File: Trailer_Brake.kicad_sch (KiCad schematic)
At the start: 11 parts, among them Q52 IRLZ44N, SW8 SW_SPST, U14 LM339

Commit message: Add files via upload
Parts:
- R201: footprint PCM_SL_Devices:Resistor_5W -> Resistor_THT:R_Axial_Power_L25.0mm_W9.0mm_P27.94mm
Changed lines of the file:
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@@
 			)
 		)
-		(property "Footprint" "PCM_SL_Devices:Resistor_5W"
+		(property "Footprint" "Resistor_THT:R_Axial_Power_L25.0mm_W9.0mm_P27.94mm"
 			(at 106.299 66.548 0)
 			(hide yes)

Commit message: Add files via upload
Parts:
- R202, R203: footprint (none) -> TRIM_3296W1103LF:TRIM_3296W1103LF
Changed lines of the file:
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@@
 			)
 		)
-		(property "Footprint" ""
+		(property "Footprint" "TRIM_3296W1103LF:TRIM_3296W1103LF"
 			(at 111.76 52.07 0)
 			(hide yes)
@@
 			)
 		)
-		(property "Footprint" ""
+		(property "Footprint" "TRIM_3296W1103LF:TRIM_3296W1103LF"
 			(at 123.19 73.66 0)
 			(hide yes)

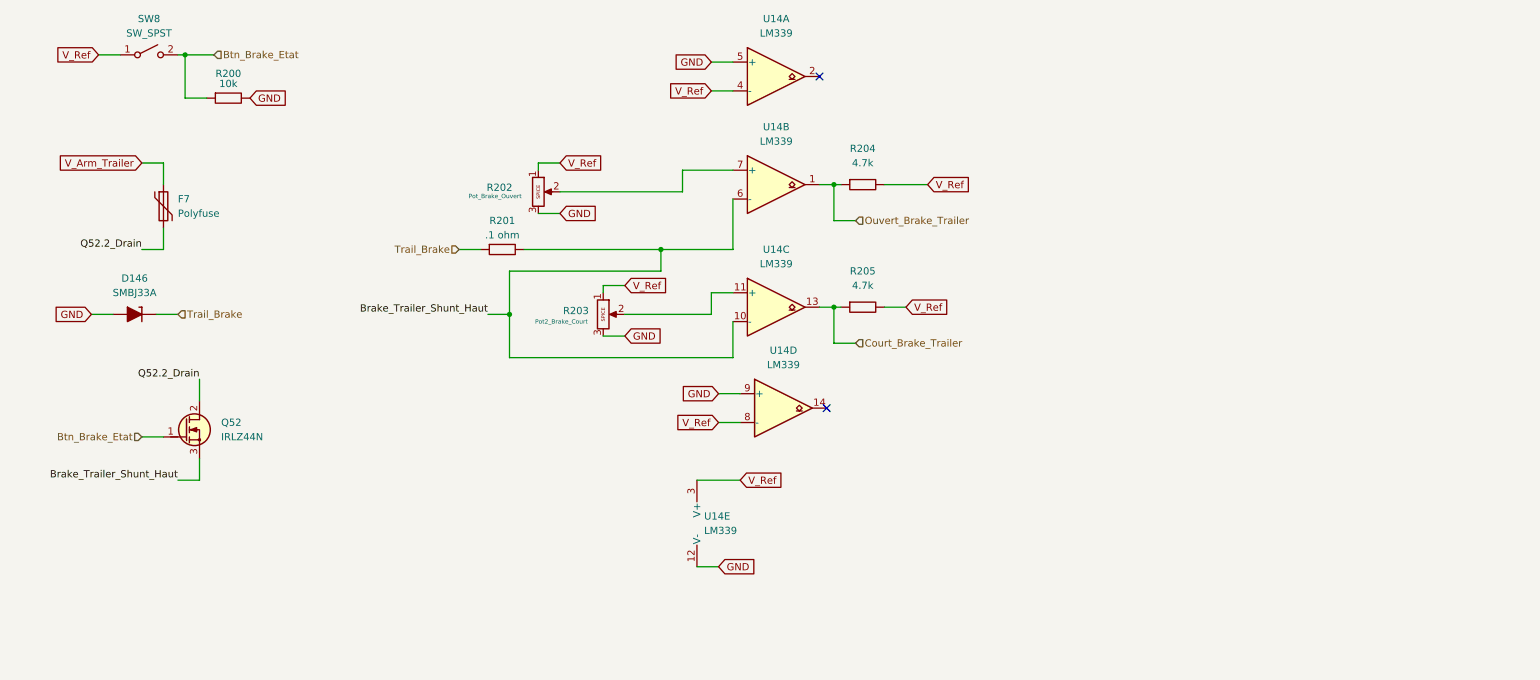
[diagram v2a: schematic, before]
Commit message: Add files via upload
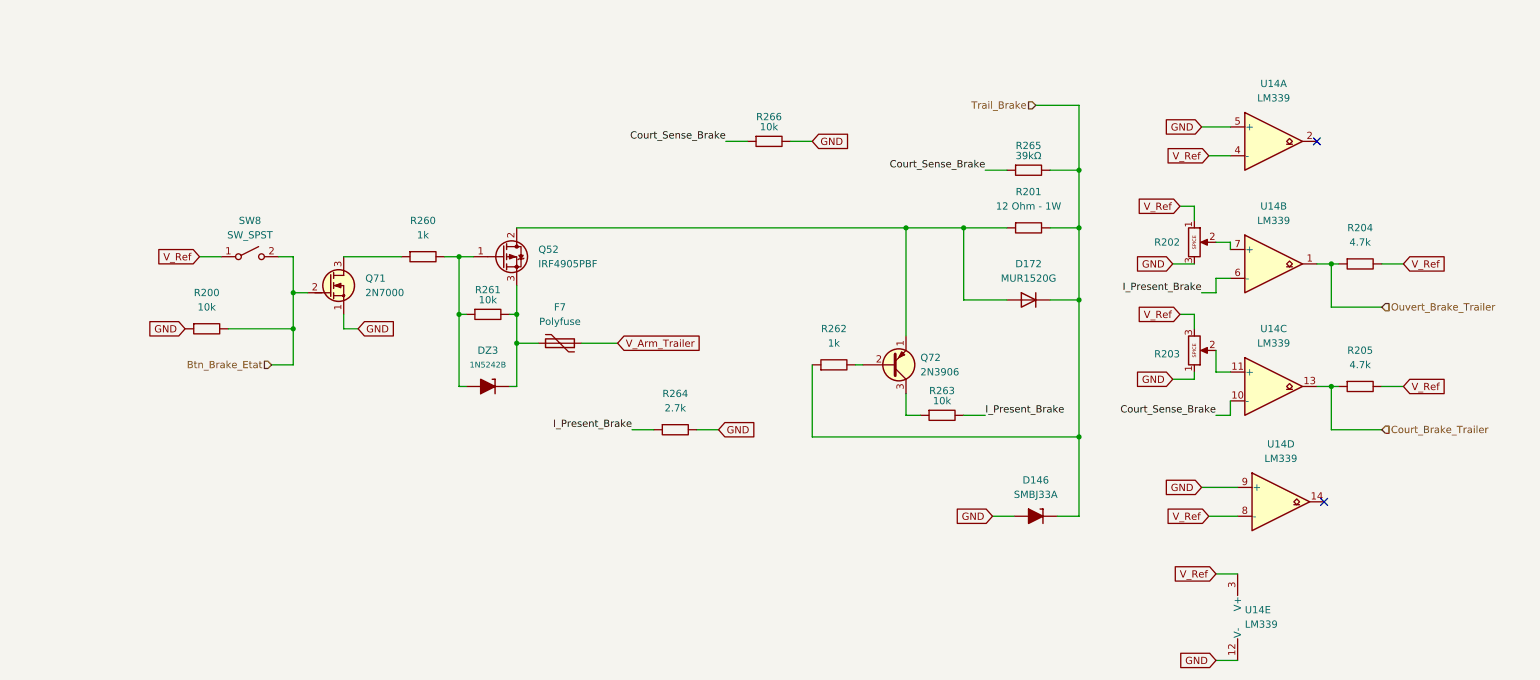
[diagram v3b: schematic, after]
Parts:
- removed Q52: IRLZ44N, PCM_Package_TO_SOT_THT_AKL:TO-220-3_Vertical_GDS, symbol PCM_Transistor_MOSFET_AKL:IRLZ44N
- removed R200: 10k, Resistor_THT:R_Axial_DIN0207_L6.3mm_D2.5mm_P10.16mm_Horizontal, symbol PCM_SL_Resistors:10k
- removed R201: .1 ohm, Resistor_THT:R_Axial_Power_L25.0mm_W9.0mm_P27.94mm, symbol PCM_SL_Resistors:4.7k
- added D172: MUR1520G, Package_TO_SOT_THT:TO-220-2_Vertical, symbol Device:D
- added DZ3: 1N5242B, PCM_Diode_THT_AKL:D_DO-35_SOD27_P7.62mm_Horizontal_Zener, symbol PCM_Diode_Zener_AKL:1N5242B
- added Q52: IRF4905PBF, Package_TO_SOT_THT:TO-220-3_Vertical, symbol Transistor_FET:IRF4905
- added Q71: 2N7000, PCM_Package_TO_SOT_THT_AKL:TO-92_Inline_Wide_SGD, symbol PCM_Transistor_MOSFET_AKL:2N7000
- added Q72: 2N3906, PCM_Package_TO_SOT_THT_AKL:TO-92_Inline_Wide_EBC, symbol PCM_Transistor_BJT_AKL:2N3906
- added R200: 10k, Resistor_THT:R_Axial_DIN0207_L6.3mm_D2.5mm_P10.16mm_Horizontal, symbol PCM_SL_Resistors:4.7k
- added R201: 12 Ohm - 1W, Resistor_THT:R_Axial_DIN0414_L11.9mm_D4.5mm_P15.24mm_Horizontal, symbol PCM_SL_Devices:Resistor_5W
- added R260, R262: 1k, Resistor_THT:R_Axial_DIN0207_L6.3mm_D2.5mm_P10.16mm_Horizontal, symbol PCM_SL_Resistors:1k
- added R261, R263, R266: 10k, Resistor_THT:R_Axial_DIN0207_L6.3mm_D2.5mm_P10.16mm_Horizontal, symbol PCM_SL_Resistors:10k
- added R264: 2.7k, Resistor_THT:R_Axial_DIN0207_L6.3mm_D2.5mm_P10.16mm_Horizontal, symbol PCM_SL_Resistors:2.7k
- added R265: 39kΩ, Resistor_THT:R_Axial_DIN0207_L6.3mm_D2.5mm_P10.16mm_Horizontal, symbol PCM_SL_Resistors:10k
- R202: Etiquette Pot_Brake_Ouvert -> (none)
- R203: Etiquette Pot2_Brake_Court -> (none)
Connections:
- net Btn_Brake_Etat: now also Q71.2 (G), R200.2
- net GND: now also R203.1, Q71.1 (S), R200.1, R264.2, R266.2; no longer R203.3
- net Trail_Brake: now also D172.1 (K), R201.2, R262.1, R265.2
- net V_Ref: now also R203.3; no longer R203.1
- net Brake_Trailer_Shunt_Haut renamed Court_Sense_Brake
- net Court_Sense_Brake: now also R265.1, R266.1; no longer U14.6 (-)
- net Q52.2_Drain: no longer names the net of F7.2
- net Q52.2_Drain: now also DZ3.1 (K), Q52.3 (S), R261.2
- new net: Q71.3 (D), R260.1
- new net: DZ3.2 (A), Q52.1 (G), R260.2, R261.1
- new net: Q72.3 (C), R263.1
- new net: Q72.2 (B), R262.2
- new net: D172.2 (A), Q52.2 (D), Q72.1 (E), R201.1
- new net I_Present_Brake: R263.2, R264.1, U14.6 (-)
